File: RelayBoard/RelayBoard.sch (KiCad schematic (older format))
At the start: 57 parts, among them J1 Micro_SD_Card, J10 Conn_01x04_Male, J11 Conn_01x04_Male, J13 Conn_01x04_Male, J2 Screw_Terminal_01x02, J3 Conn_01x04_Male, J4 Conn_01x04_Male, J5 Conn_01x04_Male, J7 SI-52008-F, J8 SI-52008-F, J9 Conn_01x04_Male, U1 STM32F745VEHx, U2 KSZ8863RLL, U3 TJA1051T-3, U4 LF33_TO252, X1 ECS-2520MV-xxx-xx

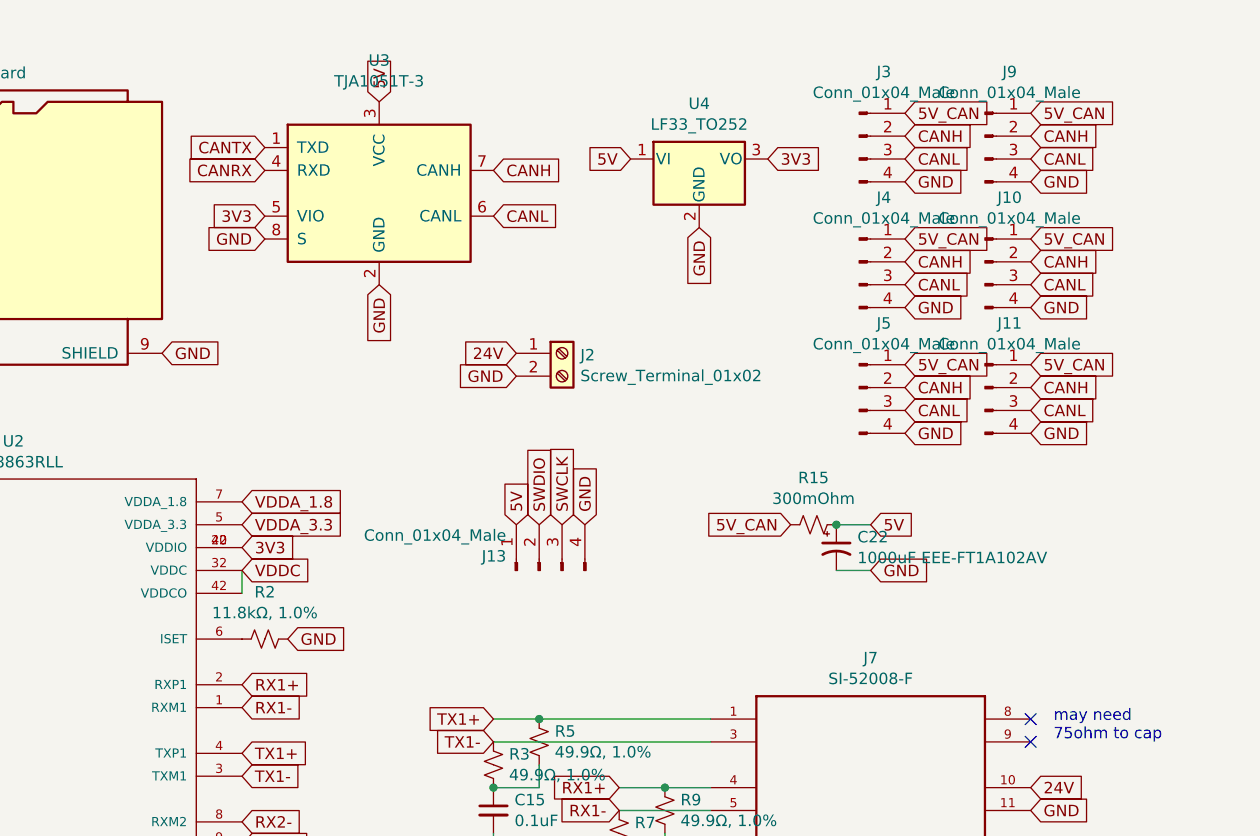
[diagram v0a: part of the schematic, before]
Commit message: ... and now it's even smaller.
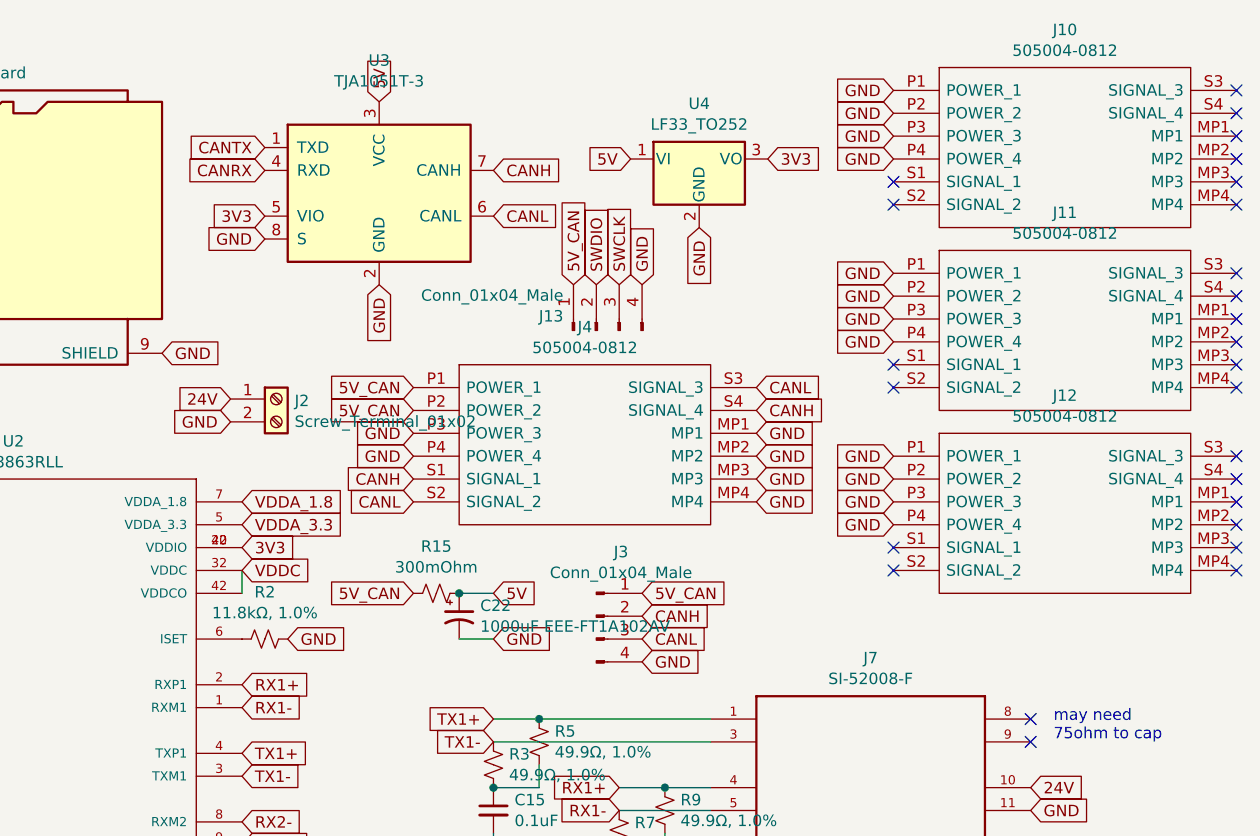
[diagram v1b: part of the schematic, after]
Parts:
- removed J10, J11, J4, J5, J9: Conn_01x04_Male, Connector_JST:JST_XH_B4B-XH-AM_1x04_P2.50mm_Vertical, symbol Connector:Conn_01x04_Male
- added J10, J11, J12, J4: 505004-0812, SamacSys_Parts:5050040812, symbol SamacSys_Parts:505004-0812
- R15: footprint (none) -> Resistor_SMD:R_0805_2012Metric_Pad1.15x1.40mm_HandSolder
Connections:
- net +5V: no longer J13.1 (Pin_1)
- net 5V_CAN: now also J13.1 (Pin_1), J4.P1 (POWER_1), J4.P2 (POWER_2)
- net CANH: now also J4.S1 (SIGNAL_1), J4.S4 (SIGNAL_4)
- net CANL: now also J4.S2 (SIGNAL_2), J4.S3 (SIGNAL_3)
- net GND: now also J10.P1 (POWER_1), J10.P2 (POWER_2), J10.P3 (POWER_3), J10.P4 (POWER_4), J11.P1 (POWER_1), J11.P2 (POWER_2), J11.P3 (POWER_3), J11.P4 (POWER_4), J12.P1 (POWER_1), J12.P2 (POWER_2), J12.P3 (POWER_3), J12.P4 (POWER_4), J4.MP1, J4.MP2, J4.MP3, J4.MP4, J4.P3 (POWER_3), J4.P4 (POWER_4)
- no-connect marks 80 -> 104
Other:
- moved on the sheet: C22, J13, J2, J3, R15
